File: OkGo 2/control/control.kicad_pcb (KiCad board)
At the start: 2 copper layers, 90.5 x 51 mm, 65 parts, among them P102 KEYSW, P103 BATT_CASE, P105 BATT, P106 ARM_LED, P108 SMA, P110 POWER_SW, P201 CH1, P202 CH2, P205 CH3, P206 CH4, Q201 BSS138BK, Q202 BSS138BK, Q203 BSS138BK, Q204 BSS138BK, U101 SWD, U102 STM32F071CBT6, U103 MEJ2S0305SC, U105 RFM95W, U106 LCD_HD44780, U107 ADP3335, Y101 8MHz

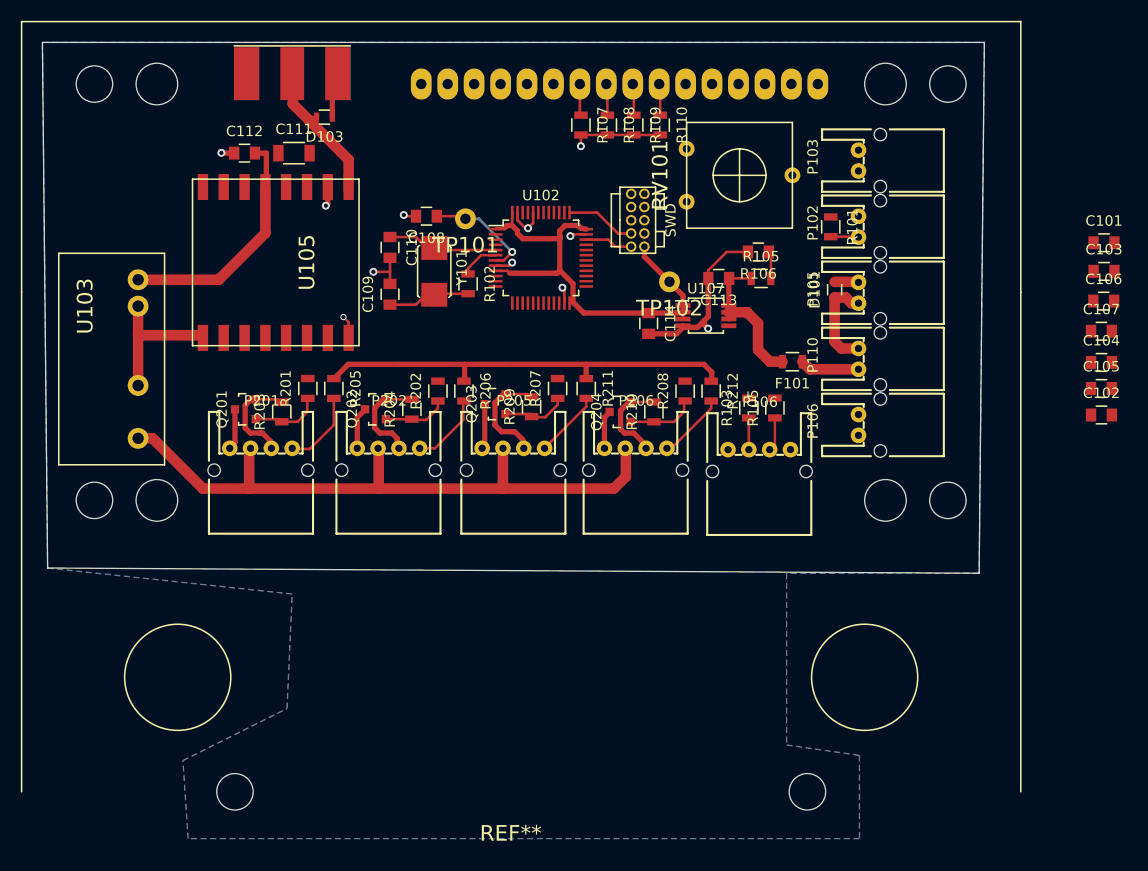
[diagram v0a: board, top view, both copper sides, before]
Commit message: Finished demo-route of control
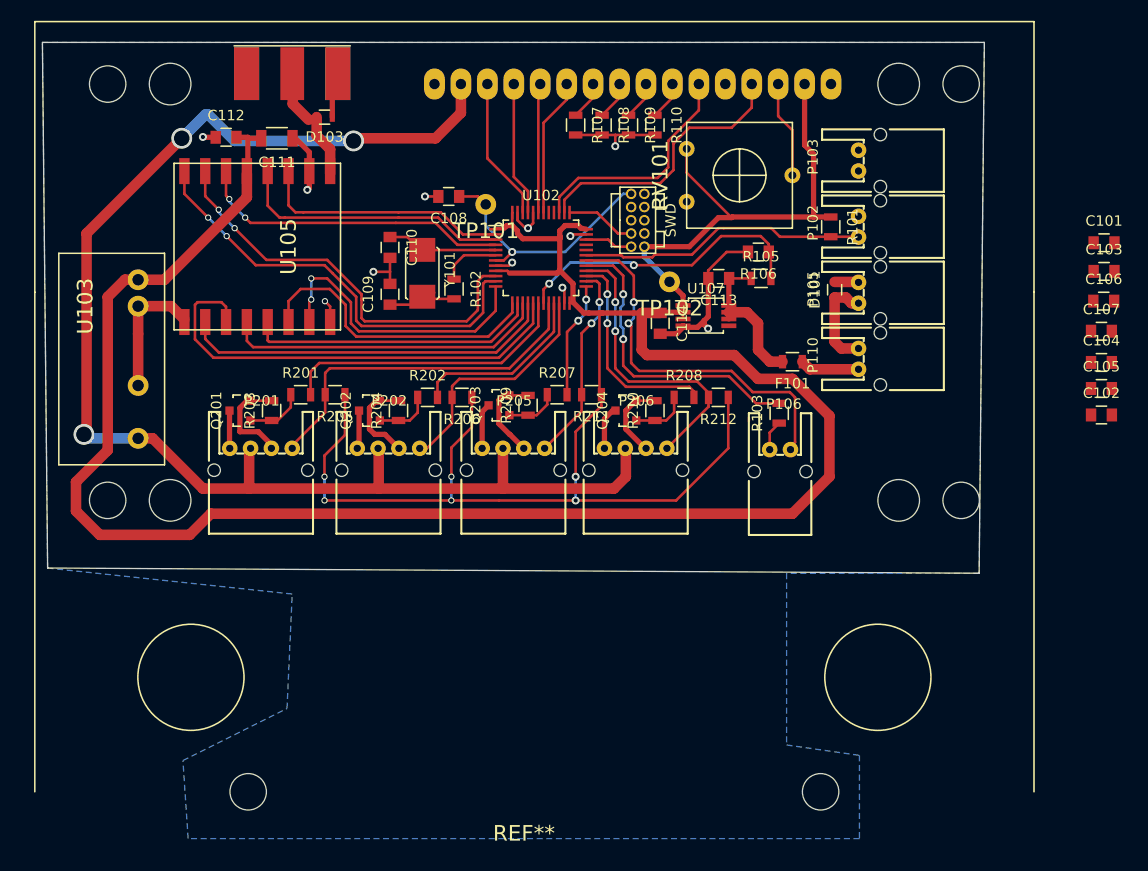
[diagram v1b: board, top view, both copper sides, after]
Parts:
- removed the P106 at (98.9, 75.1)
- removed the P106 at (105.4, 71.8)
- removed the R105 at (97.4, 71.1)
- added P106: ARM_LED, common:JST-PA-2, F.Cu at (98.9, 75.1)
- moved R103 2.96 mm to (97.8, 71.6)
- moved C108 2.86 mm to (66.0, 50.8)
- moved TP101 2.39 mm to (69.6, 51.6)
- moved C112 2.34 mm to (44.6, 45.1)
- moved U105 2.34 mm to (47.6, 55.6)
- moved C111 2.18 mm to (49.5, 45.2), turned to 180 degrees
- moved R102 1.44 mm to (66.5, 59.7)
- moved R204 1.29 mm to (61.2, 71.4)
- moved REF** 1.27 mm to (74.3, 108.0)
- moved U106 1.27 mm to (74.3, 60.0)
- moved Y101 1.16 mm to (63.5, 56.1)
- moved R202 1.16 mm to (64.0, 70.1), turned to 0 degrees
- moved C114 1.11 mm to (86.4, 63.0)
- moved R203 0.99 mm to (49.0, 71.4)
- moved R212 0.92 mm to (91.9, 70.1), turned to 180 degrees
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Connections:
- P201 pad 1: Net-(P201-Pad1) -> /controls/CH1_SW
- P202 pad 1: Net-(P202-Pad1) -> /controls/CH2_SW
- P205 pad 1: Net-(P205-Pad1) -> /controls/CH3_SW
- P206 pad 1: Net-(P206-Pad1) -> /controls/CH4_SW
- R205 pad 2: Net-(P201-Pad1) -> /controls/CH1_SW
- R206 pad 2: Net-(P202-Pad1) -> /controls/CH2_SW
- R211 pad 2: Net-(P205-Pad1) -> /controls/CH3_SW
- R212 pad 2: Net-(P206-Pad1) -> /controls/CH4_SW
- U102 pad 10: Net-(U102-Pad10) -> /RFM_DIO1
- U102 pad 11: Net-(U102-Pad11) -> /RFM_DIO2
- U102 pad 12: Net-(U102-Pad12) -> /RFM_DIO5
- U102 pad 13: Net-(U102-Pad13) -> /RFM_RESET
- U102 pad 14: Net-(U102-Pad14) -> /RFM_NSS
- U102 pad 15: Net-(U102-Pad15) -> /RFM_SCK
- U102 pad 16: Net-(U102-Pad16) -> /RFM_MISO
- U102 pad 17: Net-(U102-Pad17) -> /RFM_MOSI
- U102 pad 18: Net-(U102-Pad18) -> /controls/CH1_LED
- U102 pad 19: Net-(U102-Pad19) -> /BATT_MON
- U102 pad 2: (no net) -> /RFM_DIO3
- U102 pad 20: Net-(U102-Pad20) -> /controls/CH1_SW
- U102 pad 21: Net-(U102-Pad21) -> /controls/CH2_LED
- U102 pad 22: Net-(U102-Pad22) -> /controls/CH2_SW
- U102 pad 25: Net-(U102-Pad25) -> /controls/CH3_LED
- U102 pad 26: Net-(U102-Pad26) -> /controls/CH3_SW
- U102 pad 27: Net-(U102-Pad27) -> /controls/CH4_LED
- U102 pad 28: Net-(U102-Pad28) -> /controls/CH4_SW
- U102 pad 29: Net-(U102-Pad29) -> /ARM_LED
- U102 pad 3: Net-(U102-Pad3) -> /RFM_DIO4
- U102 pad 30: Net-(U102-Pad30) -> /DISARM_LED
- U102 pad 31: Net-(U102-Pad31) -> /ARM_SW
- U102 pad 38: Net-(U102-Pad38) -> /LCD_RS
- U102 pad 39: Net-(U102-Pad39) -> /LCD_E
- U102 pad 4: Net-(U102-Pad4) -> /RFM_DIO0
- U102 pad 42: Net-(U102-Pad42) -> /LCD_DB4
- U102 pad 43: Net-(U102-Pad43) -> /LCD_DB5
- U102 pad 45: Net-(U102-Pad45) -> /LCD_DB6
- U102 pad 46: Net-(U102-Pad46) -> /LCD_DB7
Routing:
- net +3V3: track 111.1 -> 329.6 mm, vias 0 -> 6
- net +5V: track 64.4 -> 135.3 mm, vias 0 -> 3
- net /RFM_MOSI: track 0.00 -> 44.3 mm
- net /RFM_DIO2: track 0.00 -> 41.9 mm, vias 0 -> 2
- net /RFM_DIO1: track 0.00 -> 40.0 mm, vias 0 -> 2
- net /DISARM_LED: track 0.00 -> 36.8 mm, vias 0 -> 2
- net /RFM_MISO: track 0.00 -> 36.4 mm
- net /controls/CH1_SW: track 0.00 -> 34.3 mm
- net /RFM_SCK: track 0.00 -> 31.4 mm
- net /RFM_DIO0: track 0.00 -> 30.1 mm, vias 0 -> 2
- net /ARM_LED: track 0.00 -> 29.3 mm, vias 0 -> 2
- net /controls/CH4_SW: track 0.00 -> 29.2 mm, vias 0 -> 2
- net /RFM_RESET: track 0.00 -> 28.7 mm
- net /RFM_NSS: track 0.00 -> 28.3 mm
- net /RFM_DIO5: track 0.00 -> 28.2 mm, vias 0 -> 2
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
